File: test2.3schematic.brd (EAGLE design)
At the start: 18.1 x 22.3 mm, 24 parts, among them IC1 NCS21911SN2T1G, IC2 FXLN8371QR1, IC3 MAX25210ATAB9_V+, IC4 NCS21911SN2T1G, IC5 NCS21911SN2T1G

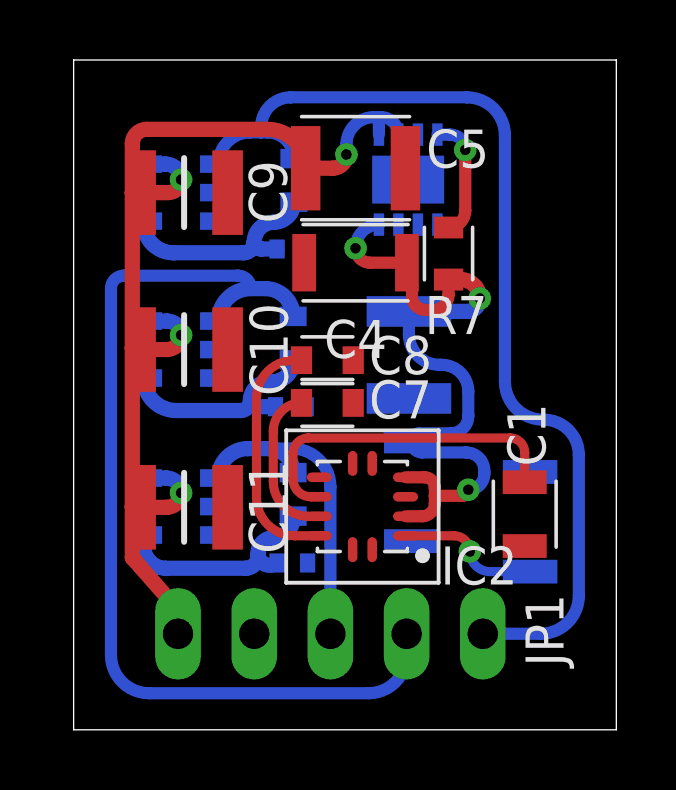
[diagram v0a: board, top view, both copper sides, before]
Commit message: Final board done, maybe for feedback from Forrest
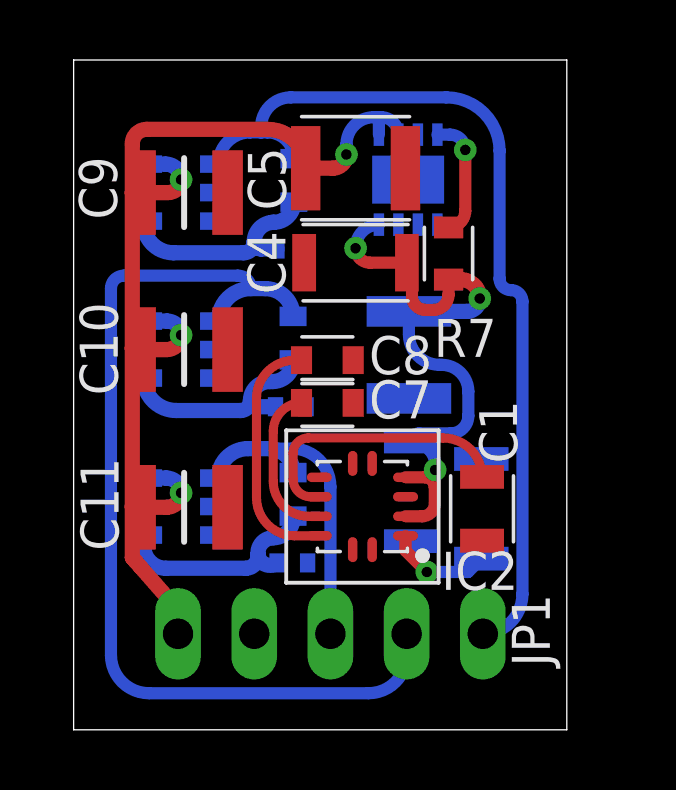
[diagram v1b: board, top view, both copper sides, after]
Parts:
- moved C6 1.68 mm to (12.9, 6.71)
- moved C1 1.43 mm to (12.9, 6.71)
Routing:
- net X_OUT: track 39.8 -> 36.7 mm
- net V_3.3V: track 24.5 -> 21.5 mm
- net Z_AXIS: track 11.1 -> 9.03 mm
- net BYP: track 4.65 -> 3.49 mm
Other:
- board size 18.1 x 22.3 mm -> 16.4 x 22.3 mm
